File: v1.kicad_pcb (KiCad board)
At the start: 4 copper layers, 223.5 x 132.1 mm, 296 parts, among them CN1 ARJM11D7-502-AB-EW2, J1 Powerpole G1377G2, J10 Barrel_Jack, J11 USB_A, J2 Conn_01x02, J3 Conn_01x02, J4 Conn_01x02, J5 Conn_01x02, J6 Conn_01x02, J7 Conn_01x02, J8 Micro_SD_Card_Det, J9 USB_B_Micro, M1 Logo_10mmx10mm, Q1 Si7141DP, Q10 Si7141DP, Q11 SI1539CDL-T1-GE3, Q12 SI1539CDL-T1-GE3, Q15 Si7141DP, Q16 SI1539CDL-T1-GE3, Q17 Si7141DP, Q18 SI1539CDL-T1-GE3, Q19 Si7141DP, Q2 SI1539CDL-T1-GE3, Q20 SI1539CDL-T1-GE3, Q21 SI1539CDL-T1-GE3, Q5 Si7141DP, Q6 SI1539CDL-T1-GE3, Q7 Si7141DP, SW1 SW_SPDT, SW2 SW_Push, T1 Transformer_SP_1S, U1 171050601, U15 MAX9612, U17 TPS3701DDCR, U18 NCP1117-3.3_TO252, U24 MAX9612, U26 TPS3701DDCR, U27 NCP1117-3.3_TO252, U28 TLV803S, U34 MAX9612, U36 TPS3701DDCR, U41 MAX9612, U43 TPS3701DDCR, U44 LT3460, U49 MAX9612, U51 TPS3701DDCR, U52 LTC2216, U53 TXS02612, U54 TE0720, U55 JTAG-SMT3, U56 TPD2S017, U57 TPS2051B, U58 TPD2S017, U59 AD5689RxCPZ, U6 MAX9612, U8 TPS3701DDCR, U9 171050601

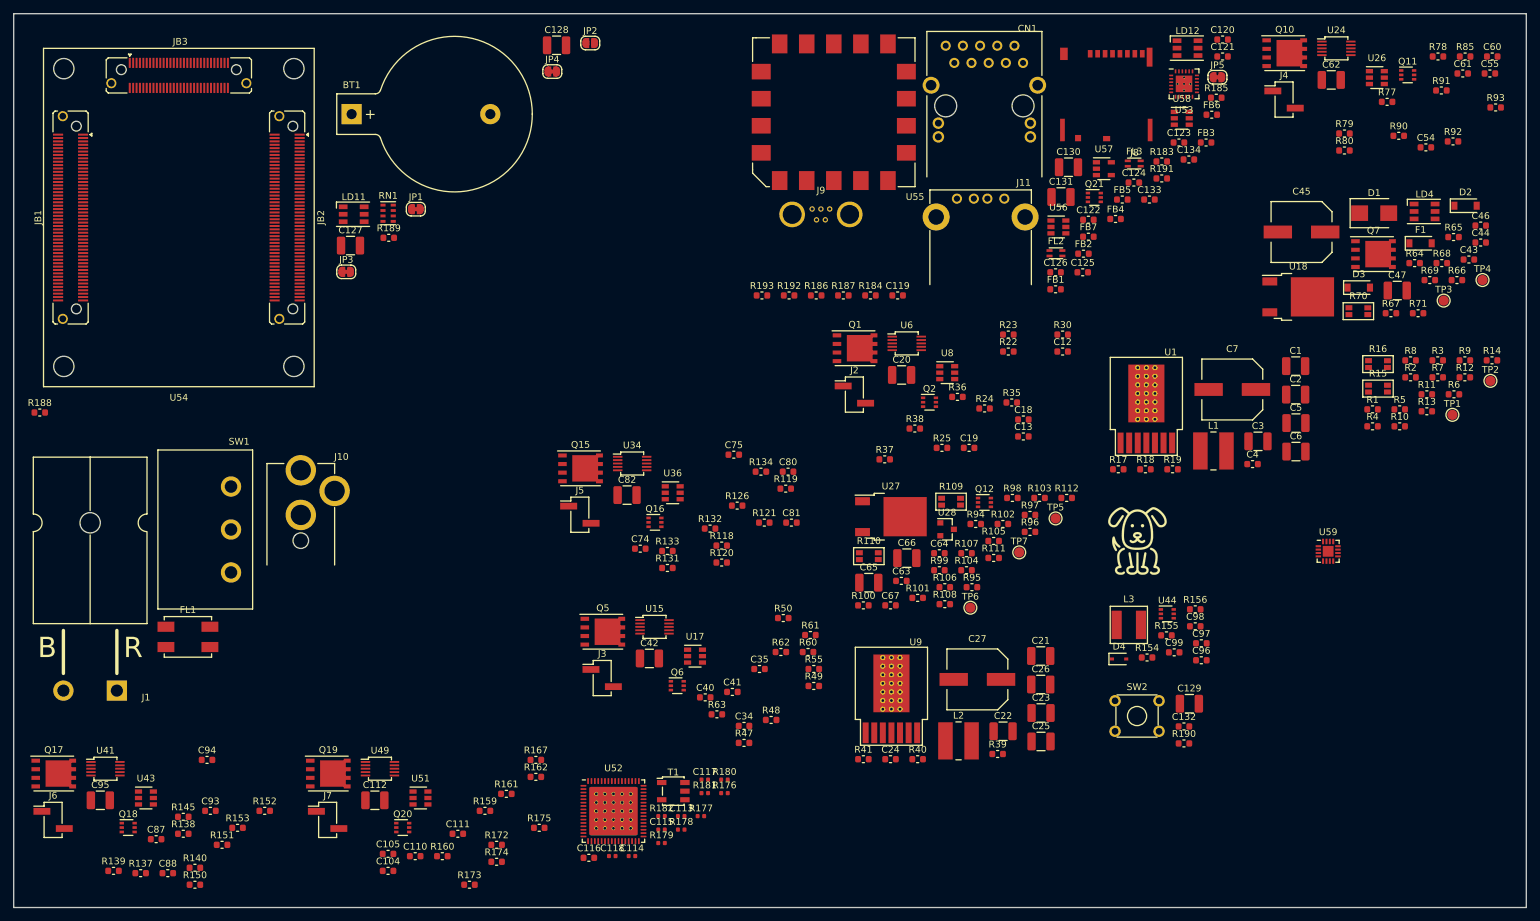
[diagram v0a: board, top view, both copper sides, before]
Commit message: muppet hadn't saved everything :(
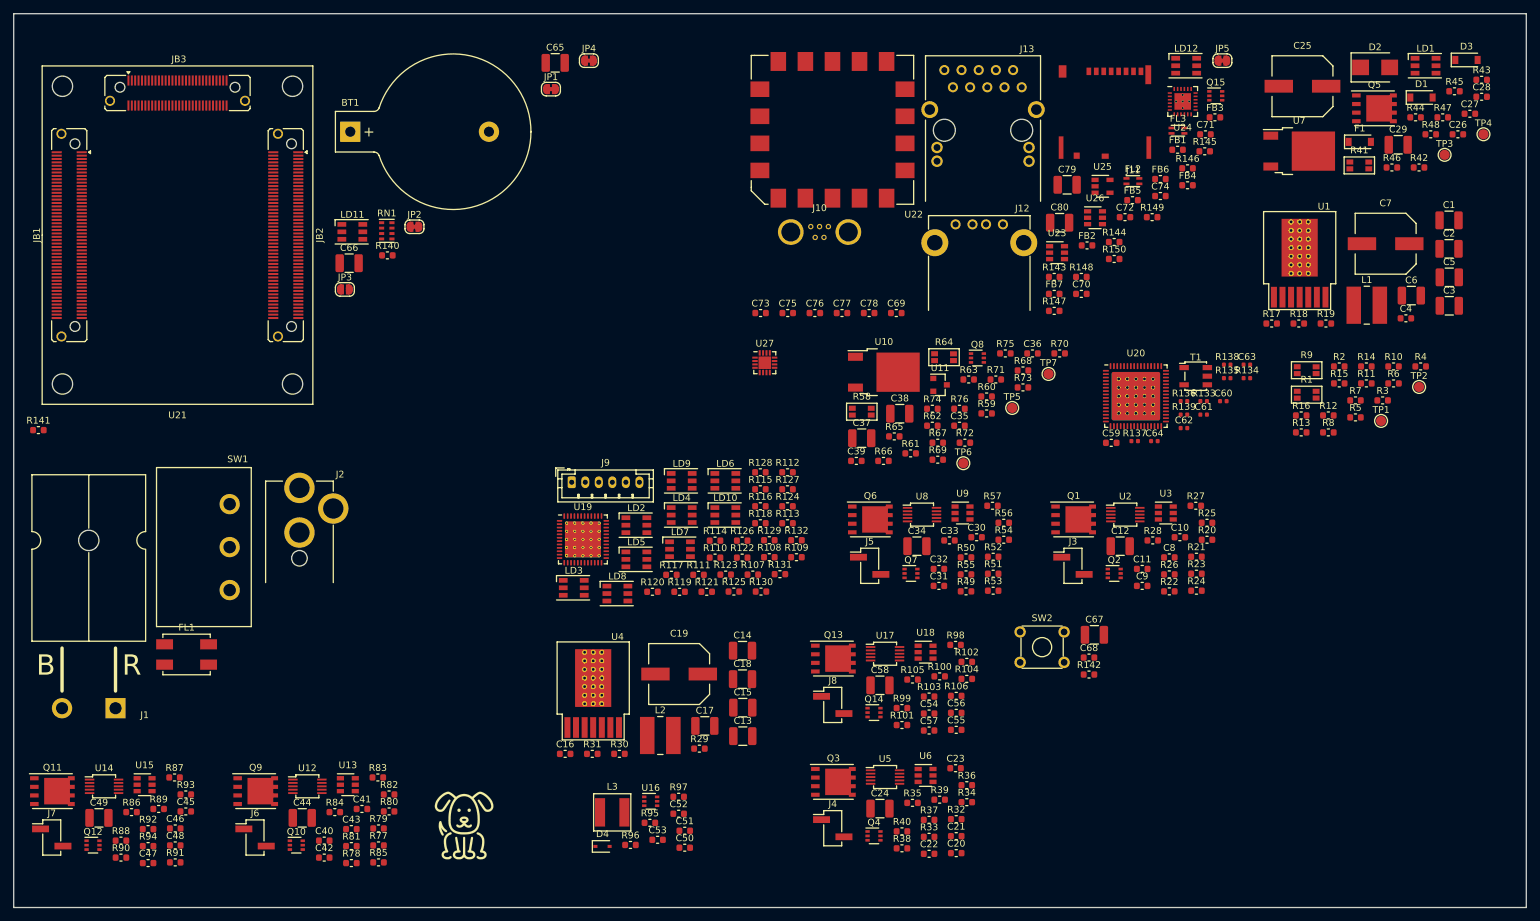
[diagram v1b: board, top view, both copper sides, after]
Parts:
- removed C104, C110, C87, C93, C96: 4u7, Capacitor_SMD:C_0603_1608Metric
- removed C105, C111, C123, C125, C126, C132, C134, C81, C88, C94: 100n, Capacitor_SMD:C_0603_1608Metric
- removed C112, C127, C128, C129, C82, C95: 22u, Capacitor_SMD:C_1210_3225Metric
- removed C113: 10n, Capacitor_SMD:C_0402_1005Metric
- removed C114: 100n, Capacitor_SMD:C_0402_1005Metric
- removed C115, C117, C118: 8p2, Capacitor_SMD:C_0402_1005Metric
- removed C116: 2u2, Capacitor_SMD:C_0603_1608Metric
- removed C119, C120, C121: 100nF, Capacitor_SMD:C_0603_1608Metric
- removed C122, C124, C133: 1u, Capacitor_SMD:C_0603_1608Metric
- removed C130, C131: 47u, Capacitor_SMD:C_1210_3225Metric
- removed C97: 47n, Capacitor_SMD:C_0603_1608Metric
- removed C98: 22p, Capacitor_SMD:C_0603_1608Metric
- removed C99: 22u, Capacitor_SMD:C_0603_1608Metric
- removed CN1: ARJM11D7-502-AB-EW2, Connector_WUT:Connector_RJ45_Magjack_Abracon_ARJM11D7-502-AB-EW2
- removed Q16, Q18, Q20, Q21: SI1539CDL-T1-GE3, Package_TO_SOT_SMD:SOT-363_SC-70-6
- removed Q17, Q19: Si7141DP, Package_SO:PowerPAK_SO-8_Single
- removed R151, R152, R173, R174, R183, R185, R190, R191: 10k, Resistor_SMD:R_0603_1608Metric
- removed R153, R154, R167, R175: 47k, Resistor_SMD:R_0603_1608Metric
- removed R155: 390k, Resistor_SMD:R_0603_1608Metric
- removed R156, R188, R192: 33k, Resistor_SMD:R_0603_1608Metric
- removed R159, R160, R161, R162: R, Resistor_SMD:R_0603_1608Metric
- removed R172: 100R, Resistor_SMD:R_0603_1608Metric
- removed R176, R177: 10R, Resistor_SMD:R_0402_1005Metric
- removed R178, R179: 35R, Resistor_SMD:R_0402_1005Metric
- removed R180, R181, R182: 5R1, Resistor_SMD:R_0402_1005Metric
- removed R184: 4k7, Resistor_SMD:R_0603_1608Metric
- removed R186, R187: 1k, Resistor_SMD:R_0603_1608Metric
- removed R189, R193: 22k, Resistor_SMD:R_0603_1608Metric
- removed U28: TLV803S, Package_TO_SOT_SMD:SOT-23
- removed U34, U41, U49: MAX9612, IC_WUT:uMAX-10_3x3mm_P0.5mm
- removed U36, U43, U51: TPS3701DDCR, Package_TO_SOT_SMD:SOT-23-6
- removed U44: LT3460, Package_TO_SOT_SMD:SOT-363_SC-70-6
- removed U52: LTC2216, IC_WUT:QFN-64-1EP_9x9mm_P0.5mm_EP7.15x7.15mm
- removed U53: TXS02612, IC_WUT:WQFN-24-1EP_4.1x4.1mm_P0.5mm_EP2.45x2.45mm
- removed U54: TE0720, IC_WUT:Trenz_TE0720
- removed U55: JTAG-SMT3, Misc_WUT:JTAG-SMT3-NC
- removed U56, U58: TPD2S017, Package_TO_SOT_SMD:SOT-23-6
- removed U57: TPS2051B, Package_TO_SOT_SMD:SOT-23-5
- removed U59: AD5689RxCPZ, Package_CSP:LFCSP-16-1EP_3x3mm_P0.5mm_EP1.854x1.854mm
- added C10: 100n, Capacitor_SMD:C_0603_1608Metric, F.Cu at (220.6, 112.9)
- added C11: 4u7, Capacitor_SMD:C_0603_1608Metric, F.Cu at (215.0, 117.6)
- added C14: 10u, Capacitor_SMD:C_1210_3225Metric, F.Cu at (156.0, 129.7)
- added C15: 10u, Capacitor_SMD:C_1210_3225Metric, F.Cu at (156.0, 138.1)
- added C16: 470n, Capacitor_SMD:C_0603_1608Metric, F.Cu at (129.8, 144.9)
- added C17: 22u, Capacitor_SMD:C_1210_3225Metric, F.Cu at (150.4, 140.8)
- added C28: 4u7, Capacitor_SMD:C_0603_1608Metric, F.Cu at (265.2, 47.8)
- added C29: 22u, Capacitor_SMD:C_1210_3225Metric, F.Cu at (252.8, 54.9)
- added C30: 4u7, Capacitor_SMD:C_0603_1608Metric, F.Cu at (190.6, 112.9)
- added C31: 100n, Capacitor_SMD:C_0603_1608Metric, F.Cu at (185.0, 120.1)
- added C32: 100n, Capacitor_SMD:C_0603_1608Metric, F.Cu at (185.0, 117.6)
- added C33: 4u7, Capacitor_SMD:C_0603_1608Metric, F.Cu at (186.5, 113.4)
- added C36: 4u7, Capacitor_SMD:C_0603_1608Metric, F.Cu at (198.8, 85.8)
- added C37: 22u, Capacitor_SMD:C_1210_3225Metric, F.Cu at (173.6, 98.3)
- added C38: 22u, Capacitor_SMD:C_1210_3225Metric, F.Cu at (179.2, 94.7)
- added C39: 100nF, Capacitor_SMD:C_0603_1608Metric, F.Cu at (172.8, 101.6)
- added C48: 4u7, Capacitor_SMD:C_0603_1608Metric, F.Cu at (72.1, 158.5)
- added C49: 22u, Capacitor_SMD:C_1210_3225Metric, F.Cu at (60.9, 154.4)
- added C50: 22p, Capacitor_SMD:C_0603_1608Metric, F.Cu at (147.4, 158.8)
- added C51: 4u7, Capacitor_SMD:C_0603_1608Metric, F.Cu at (147.4, 156.3)
- added C52: 22u, Capacitor_SMD:C_0603_1608Metric, F.Cu at (146.5, 153.8)
- added C53: 47n, Capacitor_SMD:C_0603_1608Metric, F.Cu at (143.4, 157.6)
- added C56: 100n, Capacitor_SMD:C_0603_1608Metric, F.Cu at (187.5, 138.9)
- added C57: 4u7, Capacitor_SMD:C_0603_1608Metric, F.Cu at (183.5, 141.5)
- added C58: 22u, Capacitor_SMD:C_1210_3225Metric, F.Cu at (176.3, 134.8)
- added C59: 2u2, Capacitor_SMD:C_0603_1608Metric, F.Cu at (210.4, 99.0)
- added C68: 100n, Capacitor_SMD:C_0603_1608Metric, F.Cu at (207.2, 130.7)
- added C69: 1u, Capacitor_SMD:C_0603_1608Metric, F.Cu at (178.7, 79.8)
- added C70: 100n, Capacitor_SMD:C_0603_1608Metric, F.Cu at (206.0, 77.0)
- added C71: 1u, Capacitor_SMD:C_0603_1608Metric, F.Cu at (224.4, 53.4)
- added C72: 100n, Capacitor_SMD:C_0603_1608Metric, F.Cu at (212.5, 65.6)
- added C73: 100nF, Capacitor_SMD:C_0603_1608Metric, F.Cu at (158.6, 79.8)
- added C76: 1u, Capacitor_SMD:C_0603_1608Metric, F.Cu at (166.7, 79.8)
- added C77: 100n, Capacitor_SMD:C_0603_1608Metric, F.Cu at (170.7, 79.8)
- added C78: 100n, Capacitor_SMD:C_0603_1608Metric, F.Cu at (174.7, 79.8)
- added C79: 47u, Capacitor_SMD:C_1210_3225Metric, F.Cu at (203.9, 60.8)
- added C8: 4u7, Capacitor_SMD:C_0603_1608Metric, F.Cu at (219.0, 115.9)
- added C9: 100n, Capacitor_SMD:C_0603_1608Metric, F.Cu at (215.0, 120.1)
- added J12: USB_A, Connector_WUT:USB-A_Wurth_61400416021_TH_RA, F.Cu at (190.9, 69.4)
- added J13: ARJM11D7-502-AB-EW2, Connector_WUT:Connector_RJ45_Magjack_Abracon_ARJM11D7-502-AB-EW2, F.Cu at (191.5, 52.8)
- added LD1: LED_Cree_CLX6E-FKC, LED_SMD:LED_RGB_PLCC-6, F.Cu at (256.9, 43.2)
- added LD10: LED_Cree_CLX6E-FKC, LED_SMD:LED_RGB_PLCC-6, F.Cu at (153.4, 109.6)
- added LD2: LED_Cree_CLX6E-FKC, LED_SMD:LED_RGB_PLCC-6, F.Cu at (140.3, 111.1)
- added LD3: LED_Cree_CLX6E-FKC, LED_SMD:LED_RGB_PLCC-6, F.Cu at (131.0, 120.4)
- added LD5: LED_Cree_CLX6E-FKC, LED_SMD:LED_RGB_PLCC-6, F.Cu at (140.3, 116.2)
- added LD6: LED_Cree_CLX6E-FKC, LED_SMD:LED_RGB_PLCC-6, F.Cu at (153.4, 104.6)
- added LD7: LED_Cree_CLX6E-FKC, LED_SMD:LED_RGB_PLCC-6, F.Cu at (146.7, 114.7)
- added LD8: LED_Cree_CLX6E-FKC, LED_SMD:LED_RGB_PLCC-6, F.Cu at (137.5, 121.2)
- added LD9: LED_Cree_CLX6E-FKC, LED_SMD:LED_RGB_PLCC-6, F.Cu at (147.0, 104.6)
- added Q13: Si7141DP, Package_SO:PowerPAK_SO-8_Single, F.Cu at (169.4, 130.9)
- added Q14: SI1539CDL-T1-GE3, Package_TO_SOT_SMD:SOT-363_SC-70-6, F.Cu at (175.4, 138.8)
- added Q3: Si7141DP, Package_SO:PowerPAK_SO-8_Single, F.Cu at (169.4, 149.1)
- added Q4: SI1539CDL-T1-GE3, Package_TO_SOT_SMD:SOT-363_SC-70-6, F.Cu at (175.4, 157.1)
- added Q8: SI1539CDL-T1-GE3, Package_TO_SOT_SMD:SOT-363_SC-70-6, F.Cu at (190.7, 86.4)
- added Q9: Si7141DP, Package_SO:PowerPAK_SO-8_Single, F.Cu at (84.0, 150.4)
- added R113: 7k5, Resistor_SMD:R_0603_1608Metric, F.Cu at (162.6, 110.9)
- added R114: 33k, Resistor_SMD:R_0603_1608Metric, F.Cu at (151.9, 113.4)
- added R115: 22k, Resistor_SMD:R_0603_1608Metric, F.Cu at (158.6, 105.8)
- added R116: 7k5, Resistor_SMD:R_0603_1608Metric, F.Cu at (158.6, 108.3)
- added R117: 33k, Resistor_SMD:R_0603_1608Metric, F.Cu at (145.4, 118.5)
- added R122: 7k5, Resistor_SMD:R_0603_1608Metric, F.Cu at (155.9, 115.9)
- added R123: 33k, Resistor_SMD:R_0603_1608Metric, F.Cu at (153.5, 118.4)
- added R124: 22k, Resistor_SMD:R_0603_1608Metric, F.Cu at (162.6, 108.3)
- added R125: 7k5, Resistor_SMD:R_0603_1608Metric, F.Cu at (154.7, 121.0)
- added R127: 22k, Resistor_SMD:R_0603_1608Metric, F.Cu at (162.6, 105.8)
- added R128: 33k, Resistor_SMD:R_0603_1608Metric, F.Cu at (158.6, 103.3)
- added R129: 33k, Resistor_SMD:R_0603_1608Metric, F.Cu at (159.9, 113.4)
- added R130: 4k7, Resistor_SMD:R_0603_1608Metric, F.Cu at (158.7, 121.0)
- added R135: 5R1, Resistor_SMD:R_0402_1005Metric, F.Cu at (227.6, 89.4)
- added R136: 35R, Resistor_SMD:R_0402_1005Metric, F.Cu at (221.2, 92.8)
- added R141: 22k, Resistor_SMD:R_0603_1608Metric, F.Cu at (51.9, 97.1)
- added R142: 10k, Resistor_SMD:R_0603_1608Metric, F.Cu at (207.2, 133.2)
- added R143: 10k, Resistor_SMD:R_0603_1608Metric, F.Cu at (202.0, 74.5)
- added R144: 4k7, Resistor_SMD:R_0603_1608Metric, F.Cu at (210.9, 69.3)
- added R146: 10k, Resistor_SMD:R_0603_1608Metric, F.Cu at (221.7, 58.4)
- added R147: 33k, Resistor_SMD:R_0603_1608Metric, F.Cu at (202.0, 79.5)
- added R148: 22k, Resistor_SMD:R_0603_1608Metric, F.Cu at (206.0, 74.5)
- added R149: 1k, Resistor_SMD:R_0603_1608Metric, F.Cu at (216.5, 65.6)
- added R20: 100R, Resistor_SMD:R_0603_1608Metric, F.Cu at (224.6, 113.3)
- added R21: 10k, Resistor_SMD:R_0603_1608Metric, F.Cu at (223.0, 115.8)
- added R26: 10k, Resistor_SMD:R_0603_1608Metric, F.Cu at (219.0, 118.4)
- added R27: R, Resistor_SMD:R_0603_1608Metric, F.Cu at (222.9, 108.3)
- added R28: R, Resistor_SMD:R_0603_1608Metric, F.Cu at (216.6, 113.4)
- added R29: 68k, Resistor_SMD:R_0603_1608Metric, F.Cu at (149.6, 144.2)
- added R31: 0R, Resistor_SMD:R_0603_1608Metric, F.Cu at (133.8, 144.9)
- added R32: 100R, Resistor_SMD:R_0603_1608Metric, F.Cu at (187.5, 154.6)
- added R33: 10k, Resistor_SMD:R_0603_1608Metric, F.Cu at (183.5, 157.2)
- added R34: 47k, Resistor_SMD:R_0603_1608Metric, F.Cu at (189.1, 152.1)
- added R42: 1M2, Resistor_SMD:R_0603_1608Metric, F.Cu at (255.9, 58.3)
- added R43: 10k, Resistor_SMD:R_0603_1608Metric, F.Cu at (265.2, 45.3)
- added R44: 12k, Resistor_SMD:R_0603_1608Metric, F.Cu at (255.4, 50.9)
- added R45: 33k, Resistor_SMD:R_0603_1608Metric, F.Cu at (261.2, 47.0)
- added R46: 33k, Resistor_SMD:R_0603_1608Metric, F.Cu at (251.9, 58.3)
- added R51: 47k, Resistor_SMD:R_0603_1608Metric, F.Cu at (193.0, 118.3)
- added R52: 47k, Resistor_SMD:R_0603_1608Metric, F.Cu at (193.0, 115.8)
- added R53: R, Resistor_SMD:R_0603_1608Metric, F.Cu at (193.0, 120.8)
- added R54: R, Resistor_SMD:R_0603_1608Metric, F.Cu at (194.6, 113.3)
- added R56: R, Resistor_SMD:R_0603_1608Metric, F.Cu at (194.6, 110.8)
- added R57: R, Resistor_SMD:R_0603_1608Metric, F.Cu at (192.9, 108.3)
- added R58: 10m, Resistor_WUT:R_Shunt_Vishay_WSK1206, F.Cu at (173.6, 94.4)
- added R59: 130k, Resistor_SMD:R_0603_1608Metric, F.Cu at (192.0, 94.6)
- added R72: 10k, Resistor_SMD:R_0603_1608Metric, F.Cu at (188.8, 99.0)
- added R73: 1k8, Resistor_SMD:R_0603_1608Metric, F.Cu at (197.4, 90.8)
- added R74: 22k, Resistor_SMD:R_0603_1608Metric, F.Cu at (184.0, 93.9)
- added R75: 30k, Resistor_SMD:R_0603_1608Metric, F.Cu at (194.8, 85.8)
- added R76: 1k, Resistor_SMD:R_0603_1608Metric, F.Cu at (188.0, 93.9)
- added R81: R, Resistor_SMD:R_0603_1608Metric, F.Cu at (98.2, 158.6)
- added R82: R, Resistor_SMD:R_0603_1608Metric, F.Cu at (103.7, 150.9)
- added R83: 10k, Resistor_SMD:R_0603_1608Metric, F.Cu at (102.1, 148.4)
- added R84: R, Resistor_SMD:R_0603_1608Metric, F.Cu at (95.7, 153.5)
- added R86: 100R, Resistor_SMD:R_0603_1608Metric, F.Cu at (65.7, 153.5)
- added R87: 10k, Resistor_SMD:R_0603_1608Metric, F.Cu at (72.0, 148.4)
- added R88: 47k, Resistor_SMD:R_0603_1608Metric, F.Cu at (64.1, 157.8)
- added R89: 47k, Resistor_SMD:R_0603_1608Metric, F.Cu at (69.7, 153.1)
- added U10: NCP1117-3.3_TO252, Package_TO_SOT_SMD:TO-252-2, F.Cu at (176.8, 88.5)
- added U11: TLV803S, Package_TO_SOT_SMD:SOT-23, F.Cu at (185.2, 90.4)
- added U12: MAX9612, IC_WUT:uMAX-10_3x3mm_P0.5mm, F.Cu at (91.7, 149.7)
- added U13: TPS3701DDCR, Package_TO_SOT_SMD:SOT-23-6, F.Cu at (97.6, 149.5)
- added U14: MAX9612, IC_WUT:uMAX-10_3x3mm_P0.5mm, F.Cu at (61.6, 149.7)
- added U16: LT3460, Package_TO_SOT_SMD:SOT-363_SC-70-6, F.Cu at (142.4, 151.9)
- added U19: LCMXO2-640HC-4SG48C, Package_DFN_QFN:QFN-48-1EP_7x7mm_P0.5mm_EP5.3x5.3mm_ThermalVias, F.Cu at (132.4, 113.2)
- added U2: MAX9612, IC_WUT:uMAX-10_3x3mm_P0.5mm, F.Cu at (212.5, 109.6)
- added U20: LTC2216, IC_WUT:QFN-64-1EP_9x9mm_P0.5mm_EP7.15x7.15mm, F.Cu at (214.1, 92.1)
- added U21: TE0720, IC_WUT:Trenz_TE0720, F.Cu at (72.5, 68.3)
- added U22: JTAG-SMT3, Misc_WUT:JTAG-SMT3-NC, F.Cu at (169.2, 52.7)
- added U23: TPD2S017, Package_TO_SOT_SMD:SOT-23-6, F.Cu at (202.4, 70.9)
- added U25: TPS2051B, Package_TO_SOT_SMD:SOT-23-5, F.Cu at (209.2, 61.1)
- added U3: TPS3701DDCR, Package_TO_SOT_SMD:SOT-23-6, F.Cu at (218.5, 109.3)
- added U4: 171050601, Regulator_WUT:Wurth_171050601_TO263-7EP_EP6.4x8.54mm, F.Cu at (133.9, 133.7)
- added U5: MAX9612, IC_WUT:uMAX-10_3x3mm_P0.5mm, F.Cu at (177.0, 148.4)
- added U7: NCP1117-3.3_TO252, Package_TO_SOT_SMD:TO-252-2, F.Cu at (238.2, 55.9)
- C12, C18, C34, C44: value 4u7 -> 22u; footprint Capacitor_SMD:C_0603_1608Metric -> Capacitor_SMD:C_1210_3225Metric
- C13: value 100n -> 10u; footprint Capacitor_SMD:C_0603_1608Metric -> Capacitor_SMD:C_1210_3225Metric
- C19: value 100n -> 220u; footprint Capacitor_SMD:C_0603_1608Metric -> Capacitor_WUT:Wurth_WCAP_PSHP
- C20: value 22u -> 4u7; footprint Capacitor_SMD:C_1210_3225Metric -> Capacitor_SMD:C_0603_1608Metric
- C21, C22: value 10u -> 100n; footprint Capacitor_SMD:C_1210_3225Metric -> Capacitor_SMD:C_0603_1608Metric
- C23: value 10u -> 4u7; footprint Capacitor_SMD:C_1210_3225Metric -> Capacitor_SMD:C_0603_1608Metric
- C24: value 470n -> 22u; footprint Capacitor_SMD:C_0603_1608Metric -> Capacitor_SMD:C_1210_3225Metric
- C25: value 22u -> 220u; footprint Capacitor_SMD:C_1210_3225Metric -> Capacitor_WUT:Wurth_WCAP_PSHP
- C26: value 22u -> 47n; footprint Capacitor_SMD:C_1210_3225Metric -> Capacitor_SMD:C_0603_1608Metric
- C27, C45: value 220u -> 4u7; footprint Capacitor_WUT:Wurth_WCAP_PSHP -> Capacitor_SMD:C_0603_1608Metric
- C35: value 100n -> 4u7
- C42, C47: value 22u -> 100n; footprint Capacitor_SMD:C_1210_3225Metric -> Capacitor_SMD:C_0603_1608Metric
- C43: value 47n -> 4u7
- C46: value 4u7 -> 100n
- C60, C64: value 4u7 -> 8p2; footprint Capacitor_SMD:C_0603_1608Metric -> Capacitor_SMD:C_0402_1005Metric
- C61: value 100n -> 10n; footprint Capacitor_SMD:C_0603_1608Metric -> Capacitor_SMD:C_0402_1005Metric
- C62: value 22u -> 8p2; footprint Capacitor_SMD:C_1210_3225Metric -> Capacitor_SMD:C_0402_1005Metric
- C63: value 4u7 -> 100n; footprint Capacitor_SMD:C_0603_1608Metric -> Capacitor_SMD:C_0402_1005Metric
- C67: value 100nF -> 22u; footprint Capacitor_SMD:C_0603_1608Metric -> Capacitor_SMD:C_1210_3225Metric
- C74: value 4u7 -> 100nF
- C75: value 100n -> 100nF
- C80: value 4u7 -> 47u; footprint Capacitor_SMD:C_0603_1608Metric -> Capacitor_SMD:C_1210_3225Metric
- D1: value SMAJ24A -> MM3Z15VT1G; footprint Diode_SMD:D_SMB -> Diode_SMD:D_SOD-123
- D2: value MM3Z15VT1G -> SMAJ24A; footprint Diode_SMD:D_SOD-123 -> Diode_SMD:D_SMB
- J10: value Barrel_Jack -> USB_B_Micro; footprint Connector_WUT:Barrel-Jack_Cliff_FC681478_TH -> Connector_WUT:Micro-USB_Amphenol_MUSB-K152-30_Horizontal_TH
- J11: value USB_A -> Micro_SD_Card_Det; footprint Connector_WUT:USB-A_Wurth_61400416021_TH_RA -> Connector_WUT:Micro-SD_Molex_503398-1892
- J2: value Conn_01x02 -> Barrel_Jack; footprint Connector_PinHeader_2.54mm:PinHeader_1x02_P2.54mm_Vertical_SMD_Pin1Left -> Connector_WUT:Barrel-Jack_Cliff_FC681478_TH
- J8: value Micro_SD_Card_Det -> Conn_01x02; footprint Connector_WUT:Micro-SD_Molex_503398-1892 -> Connector_PinHeader_2.54mm:PinHeader_1x02_P2.54mm_Vertical_SMD_Pin1Left
- J9: value USB_B_Micro -> Conn_01x06_Male; footprint Connector_WUT:Micro-USB_Amphenol_MUSB-K152-30_Horizontal_TH -> Connector_JST:JST_PH_B6B-PH-K_1x06_P2.00mm_Vertical
- JP2: value SolderJumper_2_Open -> SolderJumper_2_Bridged; footprint Jumper:SolderJumper-2_P1.3mm_Open_RoundedPad1.0x1.5mm -> Jumper:SolderJumper-2_P1.3mm_Bridged_RoundedPad1.0x1.5mm
- JP3: value SolderJumper_2_Bridged -> SolderJumper_2_Open; footprint Jumper:SolderJumper-2_P1.3mm_Bridged_RoundedPad1.0x1.5mm -> Jumper:SolderJumper-2_P1.3mm_Open_RoundedPad1.0x1.5mm
- Q10, Q15, Q7: value Si7141DP -> SI1539CDL-T1-GE3; footprint Package_SO:PowerPAK_SO-8_Single -> Package_TO_SOT_SMD:SOT-363_SC-70-6
- Q11, Q6: value SI1539CDL-T1-GE3 -> Si7141DP; footprint Package_TO_SOT_SMD:SOT-363_SC-70-6 -> Package_SO:PowerPAK_SO-8_Single
- R1: value 10k -> 10m; footprint Resistor_SMD:R_0603_1608Metric -> Resistor_WUT:R_Shunt_Vishay_WSK1206
- R10: value 36k5 -> 36k
- R100: value 1M2 -> 47k
- R101: value 1k8 -> 47k
- R102: value 30k -> R
- R103, R105: value 33k -> R
- R104: value 330 -> 10k
- R106: value 680 -> R
- R107: value 22k -> 7k5
- R108, R14: value 1k -> 33k
- R109: value 10m -> 22k; footprint Resistor_WUT:R_Shunt_Vishay_WSK1206 -> Resistor_SMD:R_0603_1608Metric
- R11: value 33k -> 6k8
- R110: value 50m -> 7k5; footprint Resistor_WUT:R_Shunt_Vishay_WSK1206 -> Resistor_SMD:R_0603_1608Metric
- R111: value 1R -> 33k
- R112: value 10k -> 22k
- R118, R121: value R -> 22k
- R119: value R -> 7k5
- R12: value 1k -> 430k
- R120, R140, R48: value R -> 33k
- R126: value 47k -> 33k
- R13: value 33k -> 2k26
- R131: value 100R -> 4k7
- R133: value 10k -> 5R1; footprint Resistor_SMD:R_0603_1608Metric -> Resistor_SMD:R_0402_1005Metric
- R134: value 47k -> 10R; footprint Resistor_SMD:R_0603_1608Metric -> Resistor_SMD:R_0402_1005Metric
- R137: value R -> 35R; footprint Resistor_SMD:R_0603_1608Metric -> Resistor_SMD:R_0402_1005Metric
- R138: value R -> 10R; footprint Resistor_SMD:R_0603_1608Metric -> Resistor_SMD:R_0402_1005Metric
- R139: value R -> 5R1; footprint Resistor_SMD:R_0603_1608Metric -> Resistor_SMD:R_0402_1005Metric
- R145, R30, R38, R55: value 47k -> 10k
- R15: value 10m -> 36k5; footprint Resistor_WUT:R_Shunt_Vishay_WSK1206 -> Resistor_SMD:R_0603_1608Metric
- R150: value 100R -> 1k
- R16: value 10m -> 1k; footprint Resistor_WUT:R_Shunt_Vishay_WSK1206 -> Resistor_SMD:R_0603_1608Metric
- R2: value 3k16 -> 10k
- R22, R23, R79, R80: value R -> 47k
- R3: value 36k -> 3k16
- R35: value 100R -> 47k
- R36, R37, R40, R91: value 10k -> R
- R39: value 68k -> R
- R4: value 6k8 -> 330k
- R41: value 0R -> 10m; footprint Resistor_SMD:R_0603_1608Metric -> Resistor_WUT:R_Shunt_Vishay_WSK1206
- R47: value R -> 470
- R49, R77: value R -> 100R
- R5: value 330k -> 2k74
- R50, R78: value R -> 10k
- R6: value 2k74 -> 33k
- R60: value 100R -> 2k2
- R61: value 10k -> 33k
- R62: value 10k -> 36k
- R63: value 47k -> 330
- R64: value 10k -> 50m; footprint Resistor_SMD:R_0603_1608Metric -> Resistor_WUT:R_Shunt_Vishay_WSK1206
- R65: value 1M2 -> 330k
- R66: value 12k -> 2k74
- R68: value 33k -> 44k2
- R69: value 470 -> 680
- R70: value 10m -> 1R; footprint Resistor_WUT:R_Shunt_Vishay_WSK1206 -> Resistor_SMD:R_0603_1608Metric
- R71: value 33k -> 1M2
- R8: value 430k -> 1k
- R85, R93: value 47k -> R
- R9: value 2k26 -> 10m; footprint Resistor_SMD:R_0603_1608Metric -> Resistor_WUT:R_Shunt_Vishay_WSK1206
- R90: value 100R -> R
- R94: value 130k -> R
- R95: value 2k2 -> 390k
- R96: value 36k -> 47k
- R97: value 330k -> 33k
- R98: value 2k74 -> 100R
- R99: value 44k2 -> 10k
- TP3: value 3V3 LP -> V In
- TP4: value V In -> 3V3 LP
- U15, U6: value MAX9612 -> TPS3701DDCR; footprint IC_WUT:uMAX-10_3x3mm_P0.5mm -> Package_TO_SOT_SMD:SOT-23-6
- U17, U8: value TPS3701DDCR -> MAX9612; footprint Package_TO_SOT_SMD:SOT-23-6 -> IC_WUT:uMAX-10_3x3mm_P0.5mm
- U18: value NCP1117-3.3_TO252 -> TPS3701DDCR; footprint Package_TO_SOT_SMD:TO-252-2 -> Package_TO_SOT_SMD:SOT-23-6
- U24: value MAX9612 -> TXS02612; footprint IC_WUT:uMAX-10_3x3mm_P0.5mm -> IC_WUT:WQFN-24-1EP_4.1x4.1mm_P0.5mm_EP2.45x2.45mm
- U26: value TPS3701DDCR -> TPD2S017
- U27: value NCP1117-3.3_TO252 -> AD5689RxCPZ; footprint Package_TO_SOT_SMD:TO-252-2 -> Package_CSP:LFCSP-16-1EP_3x3mm_P0.5mm_EP1.854x1.854mm
- U9: value 171050601 -> TPS3701DDCR; footprint Regulator_WUT:Wurth_171050601_TO263-7EP_EP6.4x8.54mm -> Package_TO_SOT_SMD:SOT-23-6
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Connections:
- net Net-(LD4-Pad4) renamed /Power Supply/Power Rail Management/5V_IFault
- net Net-(LD4-Pad6) renamed /Power Supply/Power Rail Management/5V_VFault
- C12 pad 1: 3V3_LP -> +3V3
- C13 pad 1: 3V3_LP -> /Power Supply/Stage 2 Regulators/12V_In
- C18 pad 1: /Power Supply/Stage 2 Regulators/3V3 Monitor/Vin -> /Power Supply/Stage 2 Regulators/5V_5A Regulator/Vout
- C19 pad 1: Net-(C19-Pad1) -> /Power Supply/Stage 2 Regulators/5V_5A Regulator/Vout
- C20 pad 1: +3V3 -> 3V3_LP
- C21 pad 1: /Power Supply/Stage 2 Regulators/12V_In -> 3V3_LP
- C23 pad 1: Net-(C22-Pad1) -> /Power Supply/Stage 2 Regulators/5V Monitor/Vin
- C24 pad 1: Net-(C24-Pad1) -> +5V
- C25 pad 1: /Power Supply/Stage 2 Regulators/5V_5A Regulator/Vout -> Net-(C25-Pad1)
- C26 pad 1: /Power Supply/Stage 2 Regulators/5V_5A Regulator/Vout -> Net-(C26-Pad1)
- C27 pad 1: /Power Supply/Stage 2 Regulators/5V_5A Regulator/Vout -> Net-(C27-Pad1)
- C34 pad 1: 3V3_LP -> /Power Supply/Stage 2 Regulators/12V_In
- C35 pad 1: 3V3_LP -> +5V
- C40 pad 1: /Power Supply/Stage 2 Regulators/5V Monitor/Vin -> 3V3_LP
- C41 pad 1: Net-(C41-Pad1) -> 3V3_LP
- C42 pad 1: +5V -> Net-(C42-Pad1)
- C43 pad 1: Net-(C43-Pad1) -> /Power Supply/Stage 3 Regulators/1V8 Monitor/Vin
- C44 pad 1: Net-(C44-Pad1) -> +1V8
- C45 pad 1: Net-(C44-Pad1) -> 3V3_LP
- C46 pad 1: Net-(C46-Pad1) -> 3V3_LP
- C47 pad 1: 3V3_LP -> Net-(C47-Pad1)
- C60 pad 1: /Power Supply/Stage 1 Regulators/12V Monitor/Vin -> Net-(C60-Pad1)
- C61 pad 1: Net-(C61-Pad1) -> GND
- C61 pad 2: GND -> Net-(C61-Pad2)
- C62 pad 1: /Power Supply/Stage 2 Regulators/12V_In -> Net-(C60-Pad1)
- C62 pad 2: GND -> Net-(C62-Pad2)
- C63 pad 1: +5V -> Net-(C61-Pad2)
- C64 pad 1: Net-(C64-Pad1) -> Net-(C62-Pad2)
- C65 pad 1: Net-(C64-Pad1) -> +3V3
- C66 pad 1: Net-(C64-Pad1) -> +3V3
- C67 pad 1: S3_PWR_ENABLE -> +3V3
- C74 pad 1: 3V3_LP -> Net-(C74-Pad1)
- C75 pad 1: 3V3_LP -> Net-(C75-Pad1)
- C80 pad 1: /Power Supply/Stage 3 Regulators/1V8 Monitor/Vin -> Net-(C79-Pad1)
- D1 pad 1: /Power Supply/Stage 1 Regulators/Vin -> Net-(C25-Pad1)
- D1 pad 2: GND -> Net-(C26-Pad1)
- D2 pad 1: Net-(C44-Pad1) -> /Power Supply/Stage 1 Regulators/Vin
- D2 pad 2: Net-(C43-Pad1) -> GND
- F1 pad 2: Net-(C46-Pad1) -> Net-(C27-Pad1)
- FB1 pad 1: +1V8 -> +3V3
- FB1 pad 2: Net-(C119-Pad1) -> Net-(FB1-Pad2)
- FB3 pad 1: +3V3 -> +1V8
- FB3 pad 2: Net-(FB3-Pad2) -> Net-(C73-Pad1)
- FB4 pad 1: +3V3 -> Net-(C71-Pad1)
- FB4 pad 2: Net-(C121-Pad1) -> Net-(FB4-Pad2)
- FB5 pad 1: Net-(C124-Pad1) -> +3V3
- FB5 pad 2: Net-(FB5-Pad2) -> Net-(C75-Pad1)
- FB6 pad 1: Net-(FB6-Pad1) -> +3V3
- FB6 pad 2: Net-(C130-Pad1) -> Net-(C76-Pad1)
- FB7 pad 1: +3V3 -> Net-(FB7-Pad1)
- FB7 pad 2: Net-(C133-Pad1) -> Net-(C79-Pad1)
- J10 pad 1: Net-(J1-Pad1) -> Net-(FB4-Pad2)
- J10 pad 2: Net-(FL1-Pad3) -> Net-(FL2-Pad2)
- J10 pad 3: (no net) -> Net-(FL2-Pad4)
- J11 pad 1: Net-(C130-Pad1) -> Net-(J11-Pad1)
- J11 pad 4: GND -> Net-(C75-Pad1)
- J11 pad 5: GND -> Net-(J11-Pad5)
- J2 pad 1: /Power Supply/Stage 2 Regulators/3V3 Monitor/Sense+ -> Net-(J1-Pad1)
- J2 pad 2: /Power Supply/Stage 2 Regulators/3V3 Monitor/Sense- -> Net-(FL1-Pad3)
- J3 pad 1: /Power Supply/Stage 2 Regulators/5V Monitor/Sense+ -> /Power Supply/Stage 2 Regulators/3V3 Monitor/Sense+
- J3 pad 2: /Power Supply/Stage 2 Regulators/5V Monitor/Sense- -> /Power Supply/Stage 2 Regulators/3V3 Monitor/Sense-
- J4 pad 1: /Power Supply/Stage 1 Regulators/12V Monitor/Sense+ -> /Power Supply/Stage 2 Regulators/5V Monitor/Sense+
- J4 pad 2: /Power Supply/Stage 1 Regulators/12V Monitor/Sense- -> /Power Supply/Stage 2 Regulators/5V Monitor/Sense-
- J5 pad 1: /Power Supply/Stage 3 Regulators/1V8 Monitor/Sense+ -> /Power Supply/Stage 1 Regulators/12V Monitor/Sense+
- J5 pad 2: /Power Supply/Stage 3 Regulators/1V8 Monitor/Sense- -> /Power Supply/Stage 1 Regulators/12V Monitor/Sense-
- J6 pad 1: /Power Supply/Stage 3 Regulators/ADC 3V3 Monitor/Sense+ -> /Power Supply/Stage 3 Regulators/1V8 Monitor/Sense+
- J6 pad 2: /Power Supply/Stage 3 Regulators/ADC 3V3 Monitor/Sense- -> /Power Supply/Stage 3 Regulators/1V8 Monitor/Sense-
- J7 pad 1: /Power Supply/Stage 3 Regulators/16V Step-up Regulator/16V_Out -> /Power Supply/Stage 3 Regulators/ADC 3V3 Monitor/Sense+
- J7 pad 2: /Power Supply/Stage 3 Regulators/16V Monitor/Sense- -> /Power Supply/Stage 3 Regulators/ADC 3V3 Monitor/Sense-
- J8 pad 1: Net-(J8-Pad1) -> /Power Supply/Stage 3 Regulators/16V Step-up Regulator/16V_Out
- J8 pad 2: Net-(J8-Pad2) -> /Power Supply/Stage 3 Regulators/16V Monitor/Sense-
- J9 pad 1: Net-(FB5-Pad2) -> /Power Supply/Power Rail Management/JTAGEN
- J9 pad 2: Net-(FL2-Pad2) -> Net-(J9-Pad2)
- J9 pad 3: Net-(FL2-Pad4) -> Net-(J9-Pad3)
- J9 pad 5: GND -> Net-(J9-Pad5)
- JP1 pad 1: /FPGA/JB1/NOSEQ -> /FPGA/JB1/JTAGMODE
- JP2 pad 1: /FPGA/JB1/EN1 -> /FPGA/JB1/NOSEQ
- JP3 pad 1: /FPGA/JB1/MODE -> /FPGA/JB1/EN1
- JP4 pad 1: /FPGA/JB1/JTAGMODE -> /FPGA/JB1/MODE
- L2 pad 2: Net-(C22-Pad1) -> Net-(C14-Pad1)
- LD4 pad 2: GND -> Net-(LD4-Pad2)
- LD4 pad 5: Net-(LD4-Pad5) -> /Power Supply/Power Rail Management/5V_OK
- Q10 pad 1: /Power Supply/Stage 1 Regulators/12V Monitor/Vin -> GND
- Q10 pad 2: /Power Supply/Stage 1 Regulators/12V Monitor/Vin -> S3_PWR_ENABLE
- Q10 pad 3: /Power Supply/Stage 1 Regulators/12V Monitor/Vin -> Net-(Q10-Pad3)
- Q10 pad 5: /Power Supply/Stage 2 Regulators/12V_In -> Net-(Q10-Pad5)
- Q11 pad 1: GND -> /Power Supply/Stage 3 Regulators/ADC 3V3 Monitor/Vin
- Q11 pad 2: S1_PWR_ENABLE -> /Power Supply/Stage 3 Regulators/ADC 3V3 Monitor/Vin
- Q11 pad 3: Net-(Q11-Pad3) -> /Power Supply/Stage 3 Regulators/ADC 3V3 Monitor/Vin
- Q11 pad 5: Net-(Q11-Pad5) -> +3.3VADC
- Q12 pad 2: /Power Supply/Stage 3 Regulators/16V_Good -> S3_PWR_ENABLE
- Q12 pad 3: /Power Supply/Stage 3 Regulators/Backlight_Enable -> Net-(Q12-Pad3)
- Q12 pad 4: 3V3_LP -> Net-(Q12-Pad4)
- Q12 pad 6: Net-(Q12-Pad5) -> Net-(Q11-Pad4)
- Q15 pad 1: /Power Supply/Stage 3 Regulators/1V8 Monitor/Vin -> GND
- Q15 pad 2: /Power Supply/Stage 3 Regulators/1V8 Monitor/Vin -> Net-(C73-Pad1)
- Q15 pad 3: /Power Supply/Stage 3 Regulators/1V8 Monitor/Vin -> Net-(C74-Pad1)
- Q15 pad 4: Net-(Q15-Pad4) -> Net-(FB1-Pad2)
- Q15 pad 5: +1V8 -> Net-(Q15-Pad5)
- Q5 pad 1: /Power Supply/Stage 2 Regulators/5V Monitor/Vin -> Net-(C25-Pad1)
- Q5 pad 2: /Power Supply/Stage 2 Regulators/5V Monitor/Vin -> Net-(C25-Pad1)
- Q5 pad 3: /Power Supply/Stage 2 Regulators/5V Monitor/Vin -> Net-(C25-Pad1)
- Q5 pad 4: Net-(Q5-Pad4) -> Net-(C26-Pad1)
- Q5 pad 5: +5V -> /Power Supply/Stage 1 Regulators/Vin
- Q6 pad 1: GND -> /Power Supply/Stage 1 Regulators/12V Monitor/Vin
- Q6 pad 2: S2_PWR_ENABLE -> /Power Supply/Stage 1 Regulators/12V Monitor/Vin
- Q6 pad 3: Net-(Q6-Pad3) -> /Power Supply/Stage 1 Regulators/12V Monitor/Vin
- Q6 pad 5: Net-(Q6-Pad5) -> /Power Supply/Stage 2 Regulators/12V_In
- Q7 pad 1: Net-(C44-Pad1) -> GND
- Q7 pad 2: Net-(C44-Pad1) -> S1_PWR_ENABLE
- Q7 pad 3: Net-(C44-Pad1) -> Net-(Q7-Pad3)
- Q7 pad 4: Net-(C43-Pad1) -> Net-(Q7-Pad4)
- Q7 pad 5: /Power Supply/Stage 1 Regulators/Vin -> Net-(Q7-Pad5)
- R1 pad 2: /Power Supply/Stage 2 Regulators/3V3_5A Regulator/FB -> /Power Supply/Stage 2 Regulators/3V3 Monitor/Sense+
- R10 pad 1: /Power Supply/Stage 2 Regulators/5V Monitor/INb -> /Power Supply/Stage 2 Regulators/5V_5A Regulator/Vout
- R10 pad 2: GND -> /Power Supply/Stage 2 Regulators/5V_5A Regulator/FB
- R100 pad 1: /Power Supply/Stage 3 Regulators/16V Monitor/Sense- -> Net-(C56-Pad1)
- R100 pad 2: /Power Supply/Stage 3 Regulators/16V Monitor/INa -> 16V_V_Good
- R101 pad 1: /Power Supply/Stage 3 Regulators/16V Monitor/INa -> 3V3_LP
- R101 pad 2: /Power Supply/Stage 3 Regulators/16V Monitor/INb -> 16V_I_Good
- R102 pad 1: /Power Supply/Stage 3 Regulators/16V Monitor/INb -> 3V3_LP
- R102 pad 2: GND -> Net-(R102-Pad2)
- R103 pad 2: /Power Supply/Stage 3 Regulators/1V8 Monitor/SetV -> Net-(R103-Pad2)
- R104 pad 1: /Power Supply/Stage 3 Regulators/1V8 Monitor/SetV -> /Power Supply/Stage 3 Regulators/Backlight_Enable
- R105 pad 1: 3V3_LP -> Net-(R102-Pad2)
- R105 pad 2: /Power Supply/Stage 3 Regulators/ADC 3V3 Monitor/SetV -> GND
- R106 pad 1: /Power Supply/Stage 3 Regulators/ADC 3V3 Monitor/SetV -> Net-(R103-Pad2)
- R107 pad 1: 3V3_LP -> Net-(LD2-Pad1)
- R107 pad 2: /Power Supply/Stage 3 Regulators/16V Monitor/SetV -> GND
- R108 pad 1: /Power Supply/Stage 3 Regulators/16V Monitor/SetV -> Net-(LD2-Pad2)
- R109 pad 1: 1V8_from_FPGA -> Net-(LD2-Pad3)
- R109 pad 2: /Power Supply/Stage 3 Regulators/1V8 Monitor/Sense+ -> GND
- R11 pad 1: 3V3_LP -> /Power Supply/Stage 2 Regulators/5V_5A Regulator/FB
- R11 pad 2: /Power Supply/Stage 2 Regulators/3V3 Monitor/SetV -> /Power Supply/Stage 2 Regulators/5V_5A Regulator/FB_Gnd
- R110 pad 1: Net-(C64-Pad1) -> Net-(LD3-Pad1)
- R110 pad 2: /Power Supply/Stage 3 Regulators/ADC 3V3 Monitor/Sense+ -> GND
- R111 pad 1: /Power Supply/Stage 3 Regulators/16V Step-up Regulator/16V_Out -> Net-(LD3-Pad2)
- R111 pad 2: /Power Supply/Stage 3 Regulators/16V Monitor/Sense- -> GND
- R112 pad 1: 3V3_LP -> Net-(LD3-Pad3)
- R112 pad 2: Net-(Q12-Pad5) -> GND
- R118 pad 1: 3V3_LP -> Net-(LD5-Pad3)
- R118 pad 2: Net-(R118-Pad2) -> GND
- R119 pad 1: Net-(R118-Pad2) -> Net-(LD6-Pad1)
- R12 pad 1: /Power Supply/Stage 2 Regulators/3V3 Monitor/SetV -> /Power Supply/Stage 2 Regulators/5V Monitor/Vin
- R12 pad 2: GND -> /Power Supply/Stage 2 Regulators/5V Monitor/INa
- R120 pad 1: 3V3_LP -> Net-(LD6-Pad2)
- R120 pad 2: Net-(R120-Pad2) -> GND
- R121 pad 1: Net-(R120-Pad2) -> Net-(LD6-Pad3)
- R126 pad 1: 3V3_LP -> Net-(LD8-Pad2)
- R126 pad 2: /Power Supply/Stage 3 Regulators/1V8 Monitor/I_Good -> GND
- R13 pad 1: 3V3_LP -> /Power Supply/Stage 2 Regulators/5V Monitor/INa
- R13 pad 2: /Power Supply/Stage 2 Regulators/5V Monitor/SetV -> /Power Supply/Stage 2 Regulators/5V Monitor/INb
- R131 pad 1: Net-(C81-Pad1) -> +3V3
- R131 pad 2: 3V3_LP -> MON_SCL
- R132 pad 1: S3_PWR_ENABLE -> /Power Supply/Power Rail Management/JTAGEN
- R133 pad 1: /Power Supply/Stage 3 Regulators/1V8 Monitor/Vin -> Net-(C59-Pad1)
- R133 pad 2: Net-(Q15-Pad4) -> Net-(R133-Pad2)
- R134 pad 1: Net-(C81-Pad1) -> Net-(C60-Pad1)
- R134 pad 2: /Power Supply/Stage 3 Regulators/1V8 Monitor/V_Good -> Net-(R134-Pad2)
- R137 pad 1: 3V3_LP -> Net-(R133-Pad2)
- R137 pad 2: Net-(R137-Pad2) -> Net-(C62-Pad2)
- R138 pad 1: Net-(R137-Pad2) -> Net-(C62-Pad2)
- R138 pad 2: GND -> Net-(R138-Pad2)
- R139 pad 1: 3V3_LP -> Net-(R139-Pad1)
- R139 pad 2: Net-(R139-Pad2) -> Net-(C62-Pad2)
- R14 pad 1: /Power Supply/Stage 2 Regulators/5V Monitor/SetV -> 3V3_LP
- R14 pad 2: GND -> /Power Supply/Stage 2 Regulators/5V Monitor/SetV
- R140 pad 1: Net-(R139-Pad2) -> +3V3
- R140 pad 2: GND -> /FPGA/JB1/JTAGMODE
- R145 pad 1: 3V3_LP -> Net-(R144-Pad2)
- R145 pad 2: /Power Supply/Stage 3 Regulators/ADC 3V3 Monitor/I_Good -> GND
- R15 pad 1: /Power Supply/Stage 2 Regulators/3V3_5A Regulator/Vout -> /Power Supply/Stage 2 Regulators/5V Monitor/INb
- R15 pad 2: /Power Supply/Stage 2 Regulators/3V3 Monitor/Sense+ -> GND
- R150 pad 2: 3V3_LP -> ~ETH_Active
- R16 pad 1: /Power Supply/Stage 2 Regulators/5V_5A Regulator/Vout -> /Power Supply/Stage 2 Regulators/5V Monitor/SetV
- R16 pad 2: /Power Supply/Stage 2 Regulators/5V Monitor/Sense+ -> GND
- R2 pad 1: /Power Supply/Stage 2 Regulators/3V3_5A Regulator/FB -> /Power Supply/Stage 2 Regulators/3V3_5A Regulator/Vout
- R2 pad 2: /Power Supply/Stage 2 Regulators/3V3_5A Regulator/FB_Gnd -> /Power Supply/Stage 2 Regulators/3V3_5A Regulator/FB
- R22 pad 1: 3V3_LP -> Net-(C10-Pad1)
- R22 pad 2: Net-(R22-Pad2) -> 3V3_V_Good
- R23 pad 1: Net-(R22-Pad2) -> 3V3_LP
- R23 pad 2: GND -> 3V3_I_Good
- R25 pad 1: Net-(R24-Pad2) -> 3V3_LP
- R25 pad 2: GND -> Net-(R25-Pad2)
- R3 pad 1: /Power Supply/Stage 2 Regulators/5V_5A Regulator/Vout -> /Power Supply/Stage 2 Regulators/3V3_5A Regulator/FB
- R3 pad 2: /Power Supply/Stage 2 Regulators/5V_5A Regulator/FB -> /Power Supply/Stage 2 Regulators/3V3_5A Regulator/FB_Gnd
- R30 pad 1: 3V3_LP -> Net-(R29-Pad2)
- R30 pad 2: /Power Supply/Stage 2 Regulators/3V3 Monitor/I_Good -> GND
- R35 pad 1: Net-(C19-Pad1) -> 3V3_LP
- R35 pad 2: 3V3_LP -> 5V_I_Good
- R36 pad 1: S2_PWR_ENABLE -> 3V3_LP
- R36 pad 2: GND -> Net-(R36-Pad2)
- R37 pad 1: /Power Supply/Stage 2 Regulators/3V3 Monitor/Vin -> 3V3_LP
- R37 pad 2: Net-(Q1-Pad4) -> Net-(R37-Pad2)
- R38 pad 1: Net-(C19-Pad1) -> S2_PWR_ENABLE
- R38 pad 2: /Power Supply/Stage 2 Regulators/3V3 Monitor/V_Good -> GND
- R39 pad 1: Net-(C22-Pad1) -> Net-(R36-Pad2)
- R39 pad 2: Net-(R39-Pad2) -> GND
- R4 pad 1: /Power Supply/Stage 2 Regulators/5V_5A Regulator/FB -> /Power Supply/Stage 2 Regulators/3V3 Monitor/Vin
- R4 pad 2: /Power Supply/Stage 2 Regulators/5V_5A Regulator/FB_Gnd -> /Power Supply/Stage 2 Regulators/3V3 Monitor/INa
- R40 pad 1: Net-(R39-Pad2) -> Net-(R37-Pad2)
- R41 pad 1: Net-(R41-Pad1) -> Net-(C25-Pad1)
- R41 pad 2: GND -> /Power Supply/Stage 1 Regulators/12V Monitor/Sense+
- R47 pad 1: 3V3_LP -> /Power Supply/Stage 1 Regulators/12V Monitor/SetV
- R47 pad 2: Net-(R47-Pad2) -> GND
- R48 pad 1: Net-(R47-Pad2) -> 3V3_LP
- R48 pad 2: GND -> Net-(LD1-Pad5)
- R49 pad 1: 3V3_LP -> Net-(C32-Pad1)
- R49 pad 2: Net-(R49-Pad2) -> 3V3_LP
- R5 pad 1: /Power Supply/Stage 2 Regulators/3V3 Monitor/Vin -> /Power Supply/Stage 2 Regulators/3V3 Monitor/INa
- R5 pad 2: /Power Supply/Stage 2 Regulators/3V3 Monitor/INa -> /Power Supply/Stage 2 Regulators/3V3 Monitor/INb
- R50 pad 1: Net-(R49-Pad2) -> /Power Supply/Stage 1 Regulators/12V Monitor/Vin
- R50 pad 2: GND -> Net-(Q6-Pad4)
- R55 pad 1: 3V3_LP -> S1_PWR_ENABLE
- R55 pad 2: /Power Supply/Stage 2 Regulators/5V Monitor/I_Good -> GND
- R6 pad 1: /Power Supply/Stage 2 Regulators/3V3 Monitor/INa -> 3V3_LP
- R6 pad 2: /Power Supply/Stage 2 Regulators/3V3 Monitor/INb -> /Power Supply/Stage 2 Regulators/3V3 Monitor/SetV
- R60 pad 1: Net-(C41-Pad1) -> /Power Supply/Stage 3 Regulators/1V8 Monitor/INa
- R60 pad 2: 3V3_LP -> /Power Supply/Stage 3 Regulators/1V8 Monitor/INb
- R61 pad 1: S2_PWR_ENABLE -> 3V3_LP
- R61 pad 2: GND -> /Power Supply/Stage 3 Regulators/1V8 Monitor/SetV
- R62 pad 1: /Power Supply/Stage 2 Regulators/5V Monitor/Vin -> /Power Supply/Stage 3 Regulators/1V8 Monitor/INb
- R62 pad 2: Net-(Q5-Pad4) -> GND
- R63 pad 1: Net-(C41-Pad1) -> /Power Supply/Stage 3 Regulators/1V8 Monitor/SetV
- R63 pad 2: /Power Supply/Stage 2 Regulators/5V Monitor/V_Good -> GND
- R64 pad 1: Net-(C43-Pad1) -> Net-(C36-Pad1)
- R64 pad 2: GND -> /Power Supply/Stage 3 Regulators/ADC 3V3 Monitor/Sense+
- R65 pad 1: /Power Supply/Stage 1 Regulators/12V Monitor/Vin -> /Power Supply/Stage 3 Regulators/ADC 3V3 Monitor/Vin
- R65 pad 2: /Power Supply/Stage 1 Regulators/12V Monitor/INa -> /Power Supply/Stage 3 Regulators/ADC 3V3 Monitor/INa
- R66 pad 1: /Power Supply/Stage 1 Regulators/12V Monitor/INa -> /Power Supply/Stage 3 Regulators/ADC 3V3 Monitor/INa
- R66 pad 2: /Power Supply/Stage 1 Regulators/12V Monitor/INb -> /Power Supply/Stage 3 Regulators/ADC 3V3 Monitor/INb
- R67 pad 1: /Power Supply/Stage 1 Regulators/12V Monitor/INb -> 3V3_LP
- R67 pad 2: GND -> /Power Supply/Stage 3 Regulators/ADC 3V3 Monitor/SetV
- R68 pad 1: 3V3_LP -> /Power Supply/Stage 3 Regulators/ADC 3V3 Monitor/INb
- R68 pad 2: /Power Supply/Stage 1 Regulators/12V Monitor/SetV -> GND
- R69 pad 1: /Power Supply/Stage 1 Regulators/12V Monitor/SetV -> /Power Supply/Stage 3 Regulators/ADC 3V3 Monitor/SetV
- R70 pad 1: Net-(C44-Pad1) -> /Power Supply/Stage 3 Regulators/16V Step-up Regulator/16V_Out
- R70 pad 2: /Power Supply/Stage 1 Regulators/12V Monitor/Sense+ -> /Power Supply/Stage 3 Regulators/16V Monitor/Sense-
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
